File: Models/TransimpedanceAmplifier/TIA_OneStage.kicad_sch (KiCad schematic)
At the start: 2 parts, among them U4 OPA828ID

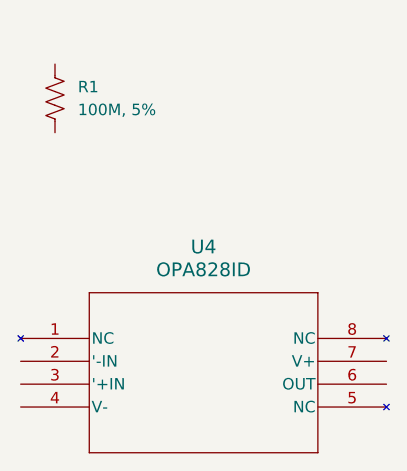
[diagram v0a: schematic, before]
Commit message: Save progress
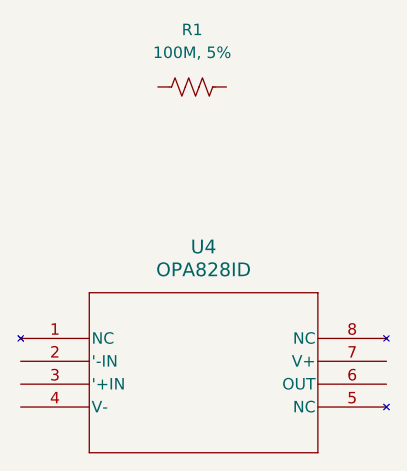
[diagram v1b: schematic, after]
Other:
- moved on the sheet: R1
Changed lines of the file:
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@@
 	(symbol
 		(lib_id "Device:R_US")
-		(at 130.81 67.31 0)
+		(at 146.05 66.04 90)
 		(unit 1)
 		(exclude_from_sim no)
@@
 		(fields_autoplaced yes)
 		(property "Reference" "R1"
-			(at 133.35 66.0399 0)
+			(at 146.05 59.69 90)
 			(effects
 				(font
 					(size 1.27 1.27)
 				)
-				(justify left)
 			)
 		)
 		(property "Value" "100M, 5%"
-			(at 133.35 68.5799 0)
+			(at 146.05 62.23 90)
 			(effects
 				(font
 					(size 1.27 1.27)
 				)
-				(justify left)
 			)
 		)
 		(property "Footprint" ""
-			(at 131.826 67.564 90)
+			(at 146.304 65.024 90)
 			(effects
 				(font
@@
 		)
 		(property "Datasheet" "~"
-			(at 130.81 67.31 0)
+			(at 146.05 66.04 0)
 			(effects
 				(font
@@
 		)
 		(property "Description" "Resistor, US symbol"
-			(at 130.81 67.31 0)
+			(at 146.05 66.04 0)
 			(effects
 				(font
@@
 		)
 		(property "Purchase Link" "https://www.digikey.com/en/products/detail/vishay-dale/CRCW0603100MJPEAHR/3232293"
-			(at 130.81 67.31 0)
+			(at 146.05 66.04 0)
 			(effects
 				(font
